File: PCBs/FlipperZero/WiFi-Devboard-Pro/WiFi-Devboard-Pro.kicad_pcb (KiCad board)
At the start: 2 copper layers, 78.5 x 20.1 mm, 46 parts, among them IC1 ESP32-WROOM-32E-N4, IC2 DMP1045U-7, IC3 AZ1117H-3.3TRE1, IC4 DMP1045U-7, IC5 DMP1045U-7, J1 3220-10-0300-00, J2 X6511WVS-08H-C60D48R2, J3 DZ254S-11-10-48, J4 Conn_01x11, J5 Conn_01x11, J6 503398-1892, U1 MMDT2907A-7-F, U2 MMDT2907A-7-F, U3 MMDT2907A-7-F

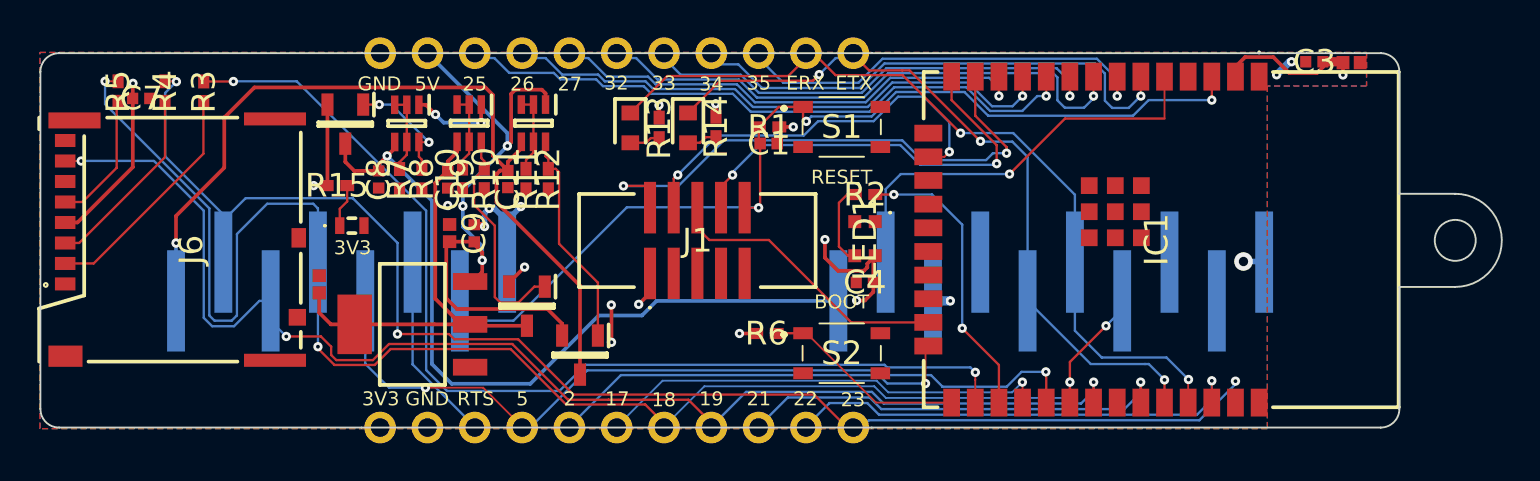
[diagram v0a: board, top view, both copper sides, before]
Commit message: Review complete, DRC done, ready for manufacturing, Tag: V0.1.0
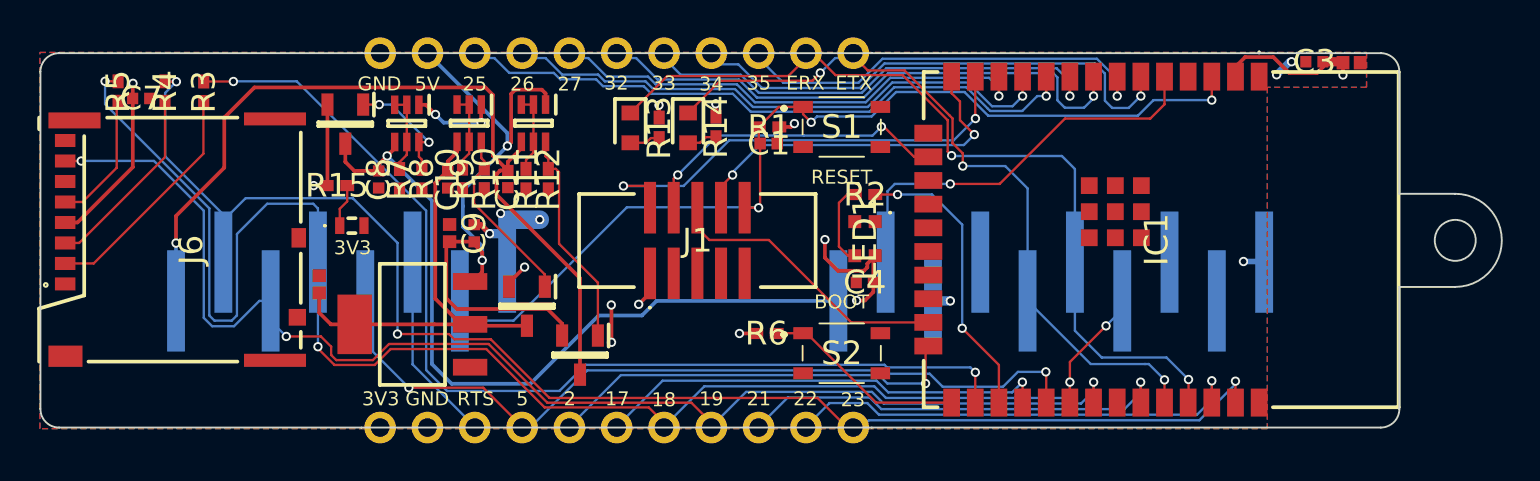
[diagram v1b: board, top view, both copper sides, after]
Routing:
- net TMS: track 29.5 -> 25.2 mm
- net TCK: track 21.6 -> 17.4 mm
- net TDI: track 23.1 -> 19.6 mm
- net Net-(IC4-Pad1): track 12.2 -> 9.64 mm
- net RX: track 43.7 -> 45.5 mm
- net GND: track 11.8 -> 13.5 mm, vias 8 -> 7
- net GPIO23: track 77.9 -> 79.0 mm
- net GPIO05: track 44.8 -> 44.2 mm
- net GPIO39: track 22.7 -> 22.1 mm
- net +5V: vias 3 -> 2
